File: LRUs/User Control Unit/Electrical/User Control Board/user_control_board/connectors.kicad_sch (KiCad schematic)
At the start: 1 part, among them J2 532611071

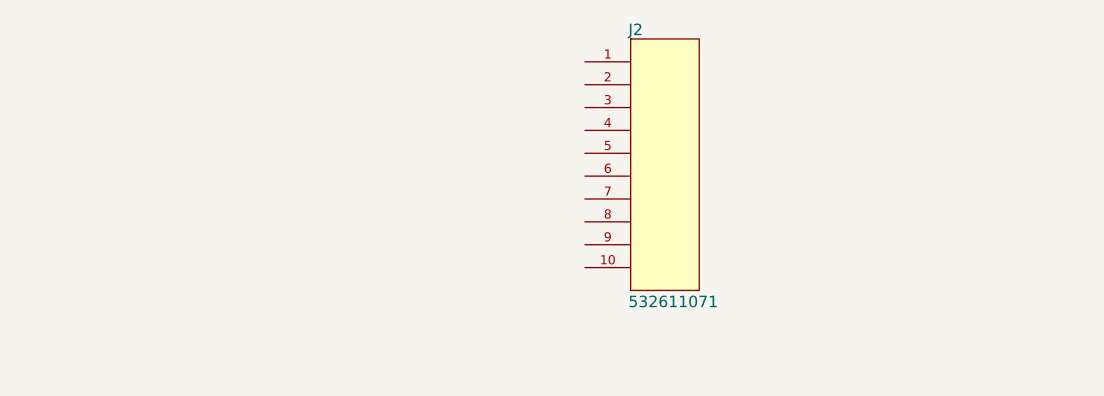
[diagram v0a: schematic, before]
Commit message: 2 pin connectors added
checking commit
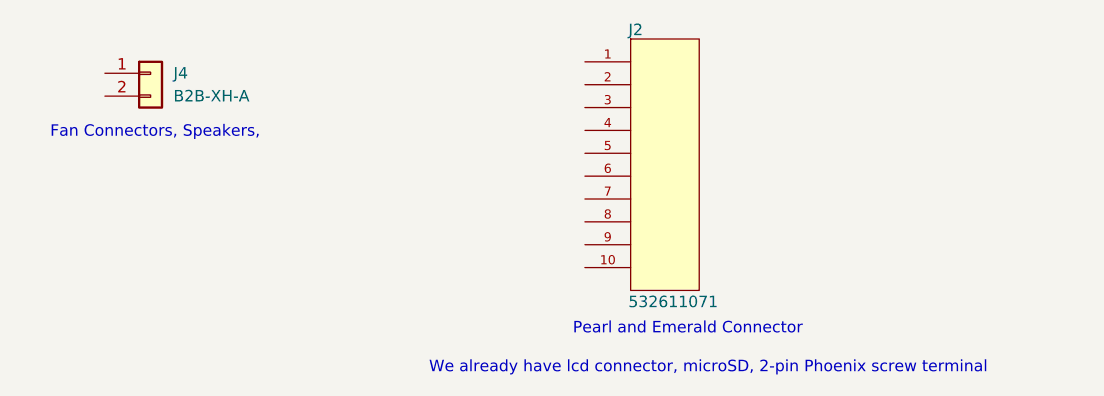
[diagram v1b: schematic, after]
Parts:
- added J4: B2B-XH-A, Connector_JST:JST_XH_B2B-XH-A_1x02_P2.50mm_Vertical, symbol Connector_Generic:Conn_01x02
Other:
- note added: "Fan Connectors, Speakers,"
- note added: "Pearl and Emerald Connector"
- note added: "We already have lcd connector, microSD, 2-pin Phoenix screw terminal"
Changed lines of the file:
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@@
 	(generator_version "10.0")
 	(paper "A4")
+	(text "Fan Connectors, Speakers, \n"
+		(exclude_from_sim no)
+		(at 180.848 49.784 0)
+		(effects
+			(font
+				(size 1.27 1.27)
+			)
+		)
+	)
+	(text "We already have lcd connector, microSD, 2-pin Phoenix screw terminal"
+		(exclude_from_sim no)
+		(at 242.316 75.946 0)
+		(effects
+			(font
+				(size 1.27 1.27)
+			)
+		)
+	)
+	(text "Pearl and Emerald Connector "
+		(exclude_from_sim no)
+		(at 240.03 71.628 0)
+		(effects
+			(font
+				(size 1.27 1.27)
+			)
+		)
+	)
+	(symbol
+		(lib_id "Connector_Generic:Conn_01x02")
+		(at 180.34 43.18 0)
+		(unit 1)
+		(body_style 1)
+		(exclude_from_sim no)
+		(in_bom yes)
+		(on_board yes)
+		(in_pos_files yes)
+		(dnp no)
+		(fields_autoplaced yes)
+		(property "Reference" "J4"
+			(at 182.88 43.1799 0)
+			(show_name no)
+			(do_not_autoplace no)
+			(effects
+				(font
+					(size 1.27 1.27)
+				)
+				(justify left)
+			)
+		)
+		(property "Value" "B2B-XH-A"
+			(at 182.88 45.7199 0)
+			(show_name no)
+			(do_not_autoplace no)
+			(effects
+				(font
+					(size 1.27 1.27)
+				)
+				(justify left)
+			)
+		)
+		(property "Footprint" "Connector_JST:JST_XH_B2B-XH-A_1x02_P2.50mm_Vertical"
+			(at 180.34 43.18 0)
+			(hide yes)
+			(show_name no)
+			(do_not_autoplace no)
+			(effects
+				(font
+					(size 1.27 1.27)
+				)
+			)
+		)
+		(property "Datasheet" ""
+			(at 180.34 43.18 0)
+			(hide yes)
+			(show_name no)
+			(do_not_autoplace no)
+			(effects
+				(font
+					(size 1.27 1.27)
+				)
+			)
+		)
+		(property "Description" "Generic connector, single row, 01x02, script generated (kicad-library-utils/schlib/autogen/connector/)"
+			(at 180.34 43.18 0)
+			(hide yes)
+			(show_name no)
+			(do_not_autoplace no)
+			(effects
+				(font
+					(size 1.27 1.27)
+				)
+			)
+		)
+		(pin "2"
+		)
+		(pin "1"
+		)
+		(instances
+			(project "user_control_board"
+				(path "/d78f77d0-5dd5-4b89-95d6-d39e93888f46"
+					(reference "J4")
+					(unit 1)
+				)
+			)
+		)
+	)
 	(symbol
 		(lib_id "symbols:532611071")

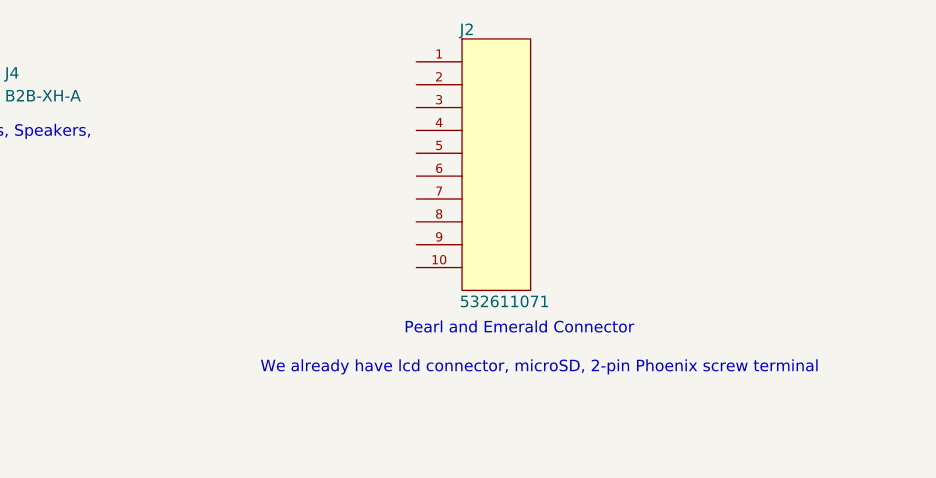
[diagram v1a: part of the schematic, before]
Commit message: DAC added Removed unnecessary modules.
Need to make custom footprint for dac.
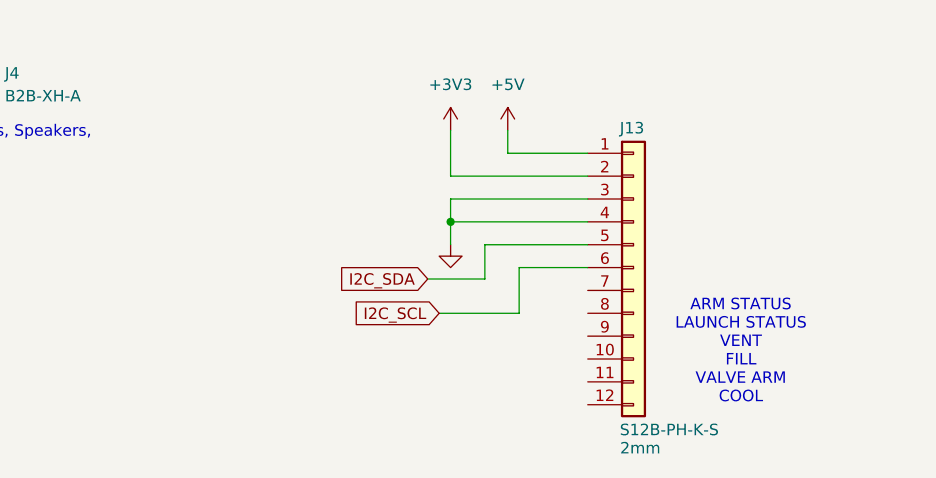
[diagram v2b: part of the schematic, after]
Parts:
- removed J2: 532611071, footprints:CONN_532610001-SD_10_MOL, symbol symbols:532611071
- added J13: S12B-PH-K-S, Connector_JST:JST_PH_S12B-PH-K_1x12_P2.00mm_Horizontal, symbol Connector_Generic:Conn_01x12
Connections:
- new net +3V3: J13.2 (Pin_2)
- new net +5V: J13.1 (Pin_1)
- new net GND: J13.3 (Pin_3), J13.4 (Pin_4)
- new net I2C_SCL: J13.6 (Pin_6)
- new net I2C_SDA: J13.5 (Pin_5)
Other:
- note added: "ARM STATUS LAUNCH STATUS VENT FILL VALVE ARM COOL"
- note removed: "Pearl and Emerald Connector"
- note removed: "We already have lcd connector, microSD, 2-pin Phoenix screw terminal"

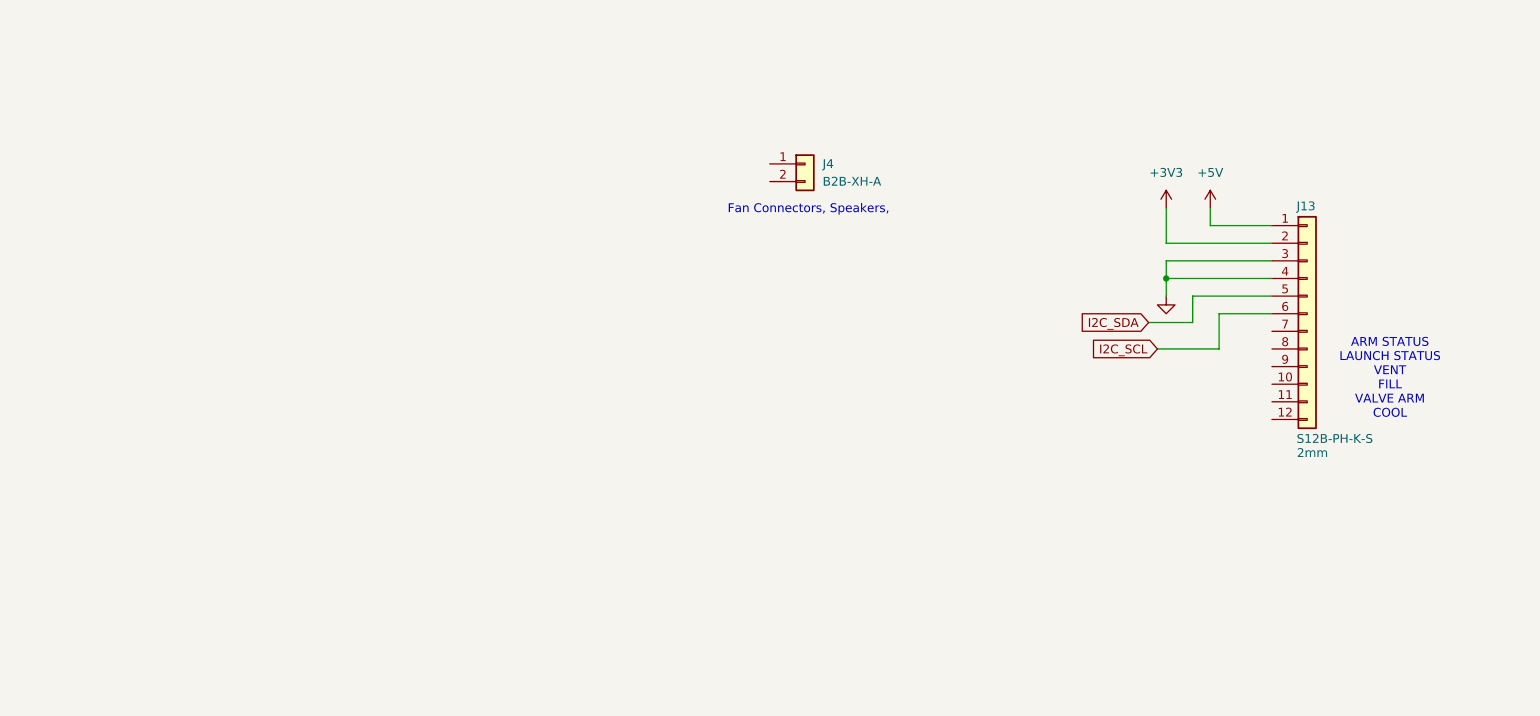
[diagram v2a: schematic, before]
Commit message: need to run DCR
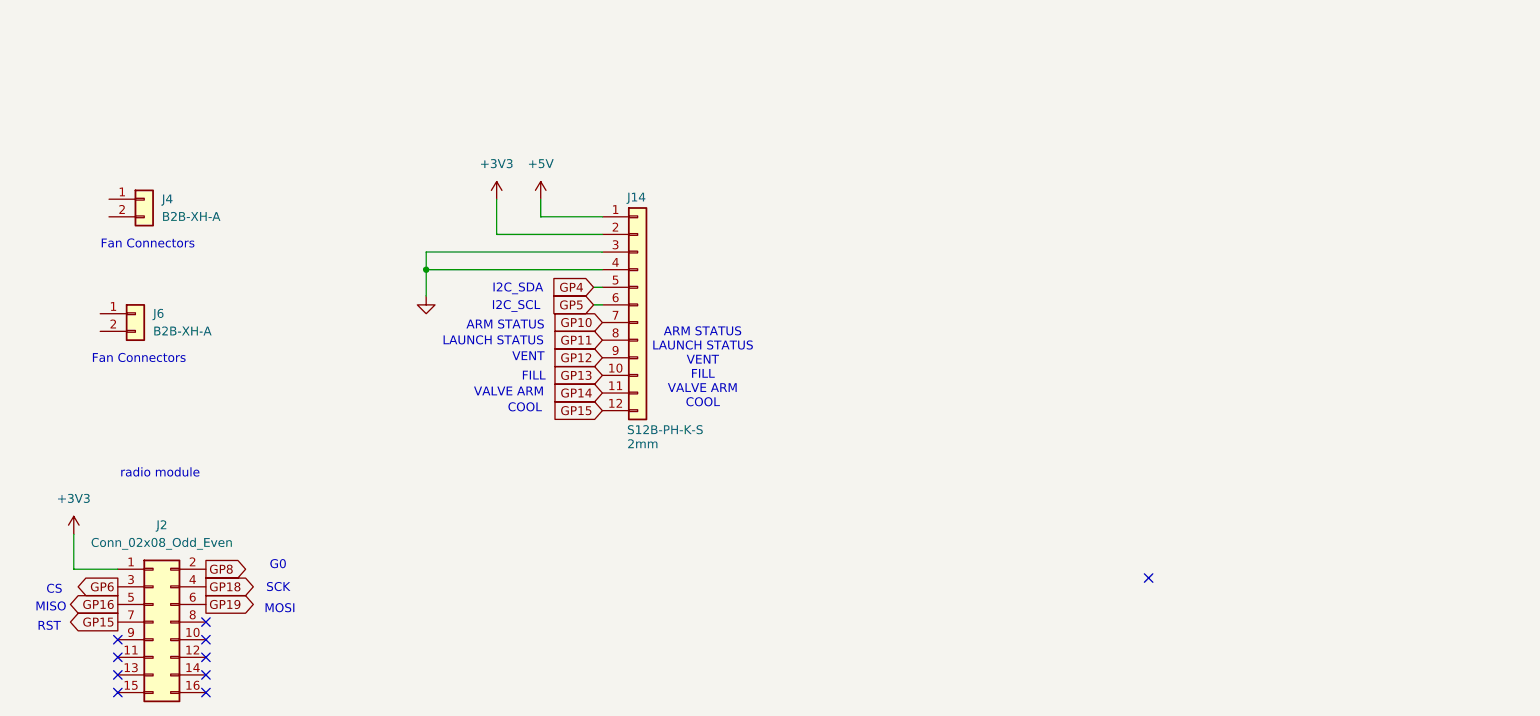
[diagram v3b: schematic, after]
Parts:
- removed J13: S12B-PH-K-S, Connector_JST:JST_PH_S12B-PH-K_1x12_P2.00mm_Horizontal, symbol Connector_Generic:Conn_01x12
- added J14: S12B-PH-K-S, Connector_JST:JST_PH_S12B-PH-K_1x12_P2.00mm_Horizontal, symbol Connector_Generic:Conn_01x12
- added J2: Conn_02x08_Odd_Even, Connector:Tag-Connect_TC2030-IDC-FP_2x03_P1.27mm_Vertical, symbol Connector_Generic:Conn_02x08_Odd_Even
- added J6: B2B-XH-A, Connector_JST:JST_XH_B2B-XH-A_1x02_P2.50mm_Vertical, symbol Connector_Generic:Conn_01x02
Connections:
- net +3V3: now also J14.2 (Pin_2), J2.1 (Pin_1)
- net +5V: now also J14.1 (Pin_1)
- net GND: now also J14.3 (Pin_3), J14.4 (Pin_4)
- new net GP10: J14.7 (Pin_7)
- new net GP11: J14.8 (Pin_8)
- new net GP12: J14.9 (Pin_9)
- new net GP13: J14.10 (Pin_10)
- new net GP14: J14.11 (Pin_11)
- new net GP15: J14.12 (Pin_12), J2.7 (Pin_7)
- new net GP16: J2.5 (Pin_5)
- new net GP18: J2.4 (Pin_4)
- new net GP19: J2.6 (Pin_6)
- new net GP4: J14.5 (Pin_5)
- new net GP5: J14.6 (Pin_6)
- new net GP6: J2.3 (Pin_3)
- new net GP8: J2.2 (Pin_2)
- no-connect marks 0 -> 10
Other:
- note added: "ARM STATUS"
- note added: "COOL"
- note added: "CS"
- note added: "FILL"
- note added: "Fan Connectors"
- note added: "G0"
- note added: "I2C_SCL"
- note added: "I2C_SDA"
- note added: "LAUNCH STATUS"
- note added: "MISO"
- note added: "MOSI"
- note added: "RST"
- note added: "SCK"
- note added: "VALVE ARM"
- note added: "VENT"
- note added: "radio module"
- note removed: "Fan Connectors, Speakers,"
- moved on the sheet: J4

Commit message: connectors and 5v buck partially done
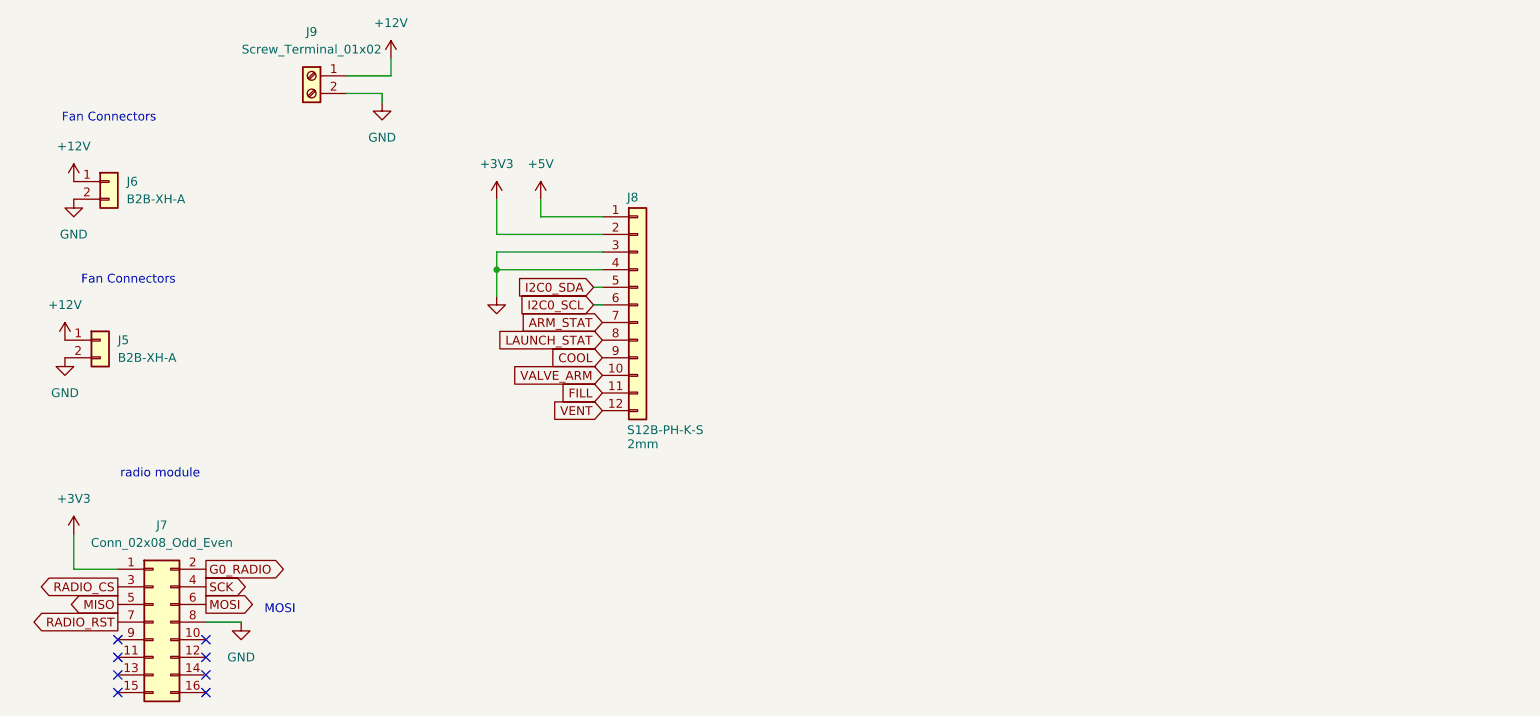
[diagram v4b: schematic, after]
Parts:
- added J9: Screw_Terminal_01x02, TerminalBlock_Phoenix:TerminalBlock_Phoenix_MPT-0,5-2-2.54_1x02_P2.54mm_Horizontal, symbol Connector:Screw_Terminal_01x02
- J7: renamed from J2; footprint Connector:Tag-Connect_TC2030-IDC-FP_2x03_P1.27mm_Vertical -> Connector_PinHeader_2.54mm:PinHeader_2x08_P2.54mm_Vertical
- renumbered J6 to J5, J4 to J6, J14 to J8
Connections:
- net GND: now also J5.2 (Pin_2), J6.2 (Pin_2), J7.8 (Pin_8), J9.2 (Pin_2)
- net +12V: now reaches J5.1 (Pin_1)
- net +12V: now also J6.1 (Pin_1), J9.1 (Pin_1)
- net GP10 renamed ARM_STAT
- net GP11 renamed LAUNCH_STAT
- net GP12 renamed COOL
- net GP13 renamed VALVE_ARM
- net GP14 renamed FILL
- net GP15 renamed RADIO_RST
- net RADIO_RST: no longer J8.12 (Pin_12)
- net GP16 renamed MISO
- net GP18 renamed SCK
- net GP19 renamed MOSI
- net GP4 renamed I2C0_SDA
- net GP5 renamed I2C0_SCL
- net GP6 renamed RADIO_CS
- net GP8 renamed G0_RADIO
- new net VENT: J8.12 (Pin_12)
- no-connect marks 10 -> 8
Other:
- note removed: "ARM STATUS"
- note removed: "ARM STATUS LAUNCH STATUS VENT FILL VALVE ARM COOL"
- note removed: "COOL"
- note removed: "CS"
- note removed: "FILL"
- note removed: "G0"
- note removed: "I2C_SCL"
- note removed: "I2C_SDA"
- note removed: "LAUNCH STATUS"
- note removed: "MISO"
- note removed: "RST"
- note removed: "SCK"
- note removed: "VALVE ARM"
- note removed: "VENT"
- moved on the sheet: J5, J6
